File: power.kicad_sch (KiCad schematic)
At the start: 8 parts, among them U3 TPS63900

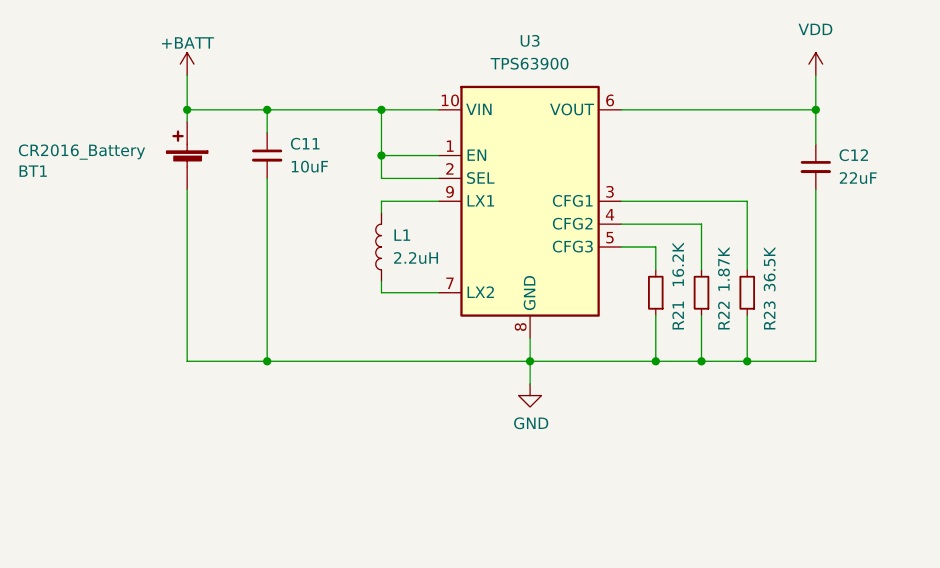
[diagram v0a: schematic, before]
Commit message: review
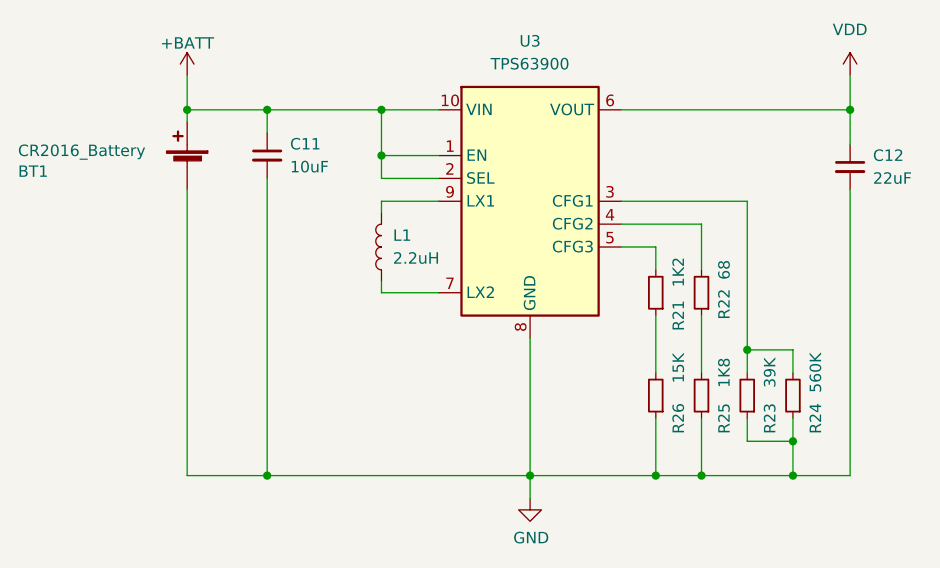
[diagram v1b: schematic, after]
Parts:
- added R24: 560K, Resistor_SMD:R_0603_1608Metric_Pad0.98x0.95mm_HandSolder, symbol Device:R_Small
- added R25: 1K8, Resistor_SMD:R_0603_1608Metric_Pad0.98x0.95mm_HandSolder, symbol Device:R_Small
- added R26: 15K, Resistor_SMD:R_0603_1608Metric_Pad0.98x0.95mm_HandSolder, symbol Device:R_Small
- R21: value 16.2K -> 1K2
- R22: value 1.87K -> 68
- R23: value 36.5K -> 39K
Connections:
- net GND: now also R24.1, R25.1, R26.1; no longer R21.1, R22.1
- net at R23.2, U3.3 (CFG1): now also R24.2
- new net: R22.1, R25.2
- new net: R21.1, R26.2
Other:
- moved on the sheet: C12, R23
